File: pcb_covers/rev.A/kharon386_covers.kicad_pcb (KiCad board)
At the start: 2 copper layers, 134.6 x 63 mm, 2 parts

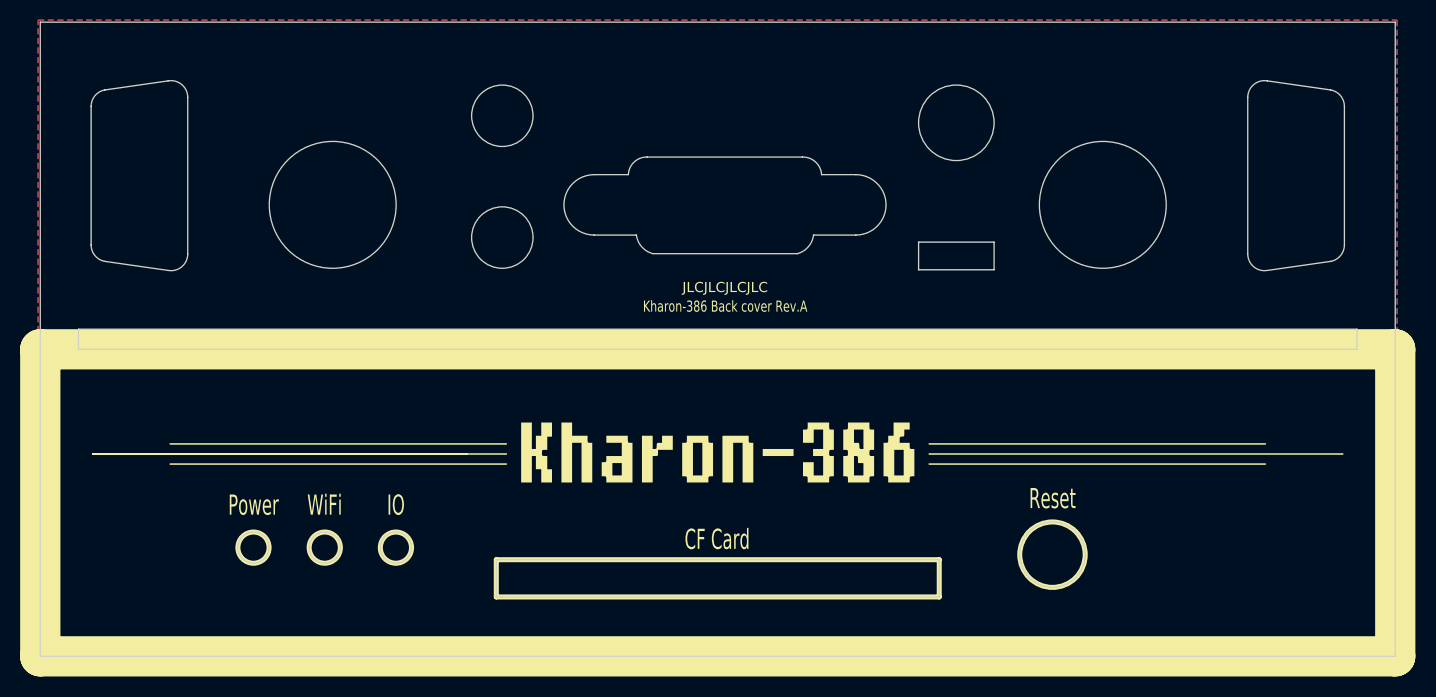
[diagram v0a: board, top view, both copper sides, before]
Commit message: pcb rev.A final version
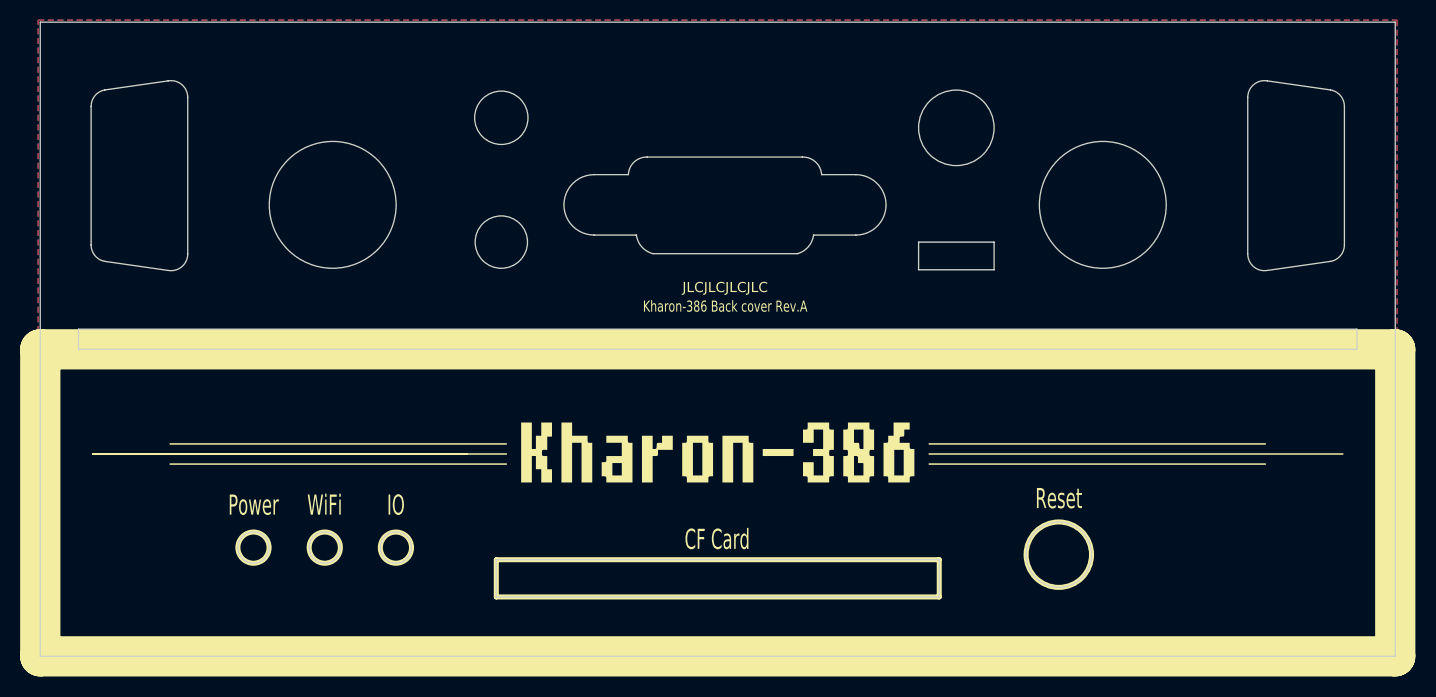
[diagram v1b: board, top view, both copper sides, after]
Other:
- outline, holes or cut-outs redrawn
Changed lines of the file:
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@@
   (gr_line (start 132.217828 76.65) (end 135.617828 76.65) (layer "B.SilkS") (width 0.5))
   (gr_arc (start 158.217828 76.65) (mid 161.21783 79.65) (end 158.217828 82.65) (layer "B.SilkS") (width 0.5))
-  (gr_circle (center 123.1 70.8) (end 126.15 70.8) (layer "B.SilkS") (width 0.5) (fill none))
+  (gr_circle (center 123 71) (end 125.65 71) (layer "B.SilkS") (width 0.5) (fill none))
   (gr_line (start 197.14969 84.529483) (end 197.14969 68.970509) (layer "B.SilkS") (width 0.5))
   (gr_arc (start 197.14969 68.970509) (mid 197.742659 67.698865) (end 199.097944 67.33573) (layer "B.SilkS") (width 0.5))
   (gr_arc (start 82.25 69.869781) (mid 82.638365 68.802753) (end 83.621743 68.235001) (layer "B.SilkS") (width 0.5))
-  (gr_circle (center 168.2 71.5) (end 171.95 71.5) (layer "B.SilkS") (width 0.5) (fill none))
+  (gr_circle (center 168.2 72) (end 171.95 72) (layer "B.SilkS") (width 0.5) (fill none))
   (gr_line (start 83.621744 85.265) (end 89.901744 86.164268) (layer "B.SilkS") (width 0.5))
-  (gr_circle (center 123.1 82.9) (end 126.15 82.9) (layer "B.SilkS") (width 0.5) (fill none))
+  (gr_circle (center 123 83.35) (end 125.6 83.35) (layer "B.SilkS") (width 0.5) (fill none))
   (gr_line (start 137.492828 74.9) (end 152.907172 74.9) (layer "B.SilkS") (width 0.5))
   (gr_line (start 138.053367 84.5) (end 152.417831 84.499999) (layer "B.SilkS") (width 0.5))
@@
   (gr_arc (start 205.377947 68.234995) (mid 206.361339 68.802744) (end 206.74969 69.869777) (layer "B.SilkS") (width 0.5))
   (gr_line (start 165.5 103.4) (end 198.9 103.4) (layer "F.SilkS") (width 0.15))
-  (gr_circle (center 177.75 114.4) (end 181 114.4) (layer "F.SilkS") (width 0.5) (fill none))
+  (gr_circle (center 178.38 114.4) (end 181.63 114.4) (layer "F.SilkS") (width 0.5) (fill none))
   (gr_line (start 123.5 104.4) (end 82.4 104.4) (layer "F.SilkS") (width 0.15))
   (gr_rect (start 77.2 94) (end 211.8 124.5) (layer "F.SilkS") (width 4) (fill none))
@@
   (gr_line (start 94.5 75.4) (end 194.5 75.4) (layer "Eco1.User") (width 0.015))
   (gr_circle (center 201.95 89.235) (end 203.35 89.235) (layer "Eco1.User") (width 0.1) (fill none))
-  (gr_circle (center 123.1 70.8) (end 126.15 70.8) (layer "Edge.Cuts") (width 0.1) (fill none))
+  (gr_circle (center 123 71) (end 125.65 71) (layer "Edge.Cuts") (width 0.1) (fill none))
   (gr_arc (start 197.14969 68.970509) (mid 197.742659 67.698865) (end 199.097944 67.33573) (layer "Edge.Cuts") (width 0.1))
   (gr_arc (start 83.621743 85.265001) (mid 82.638365 84.697247) (end 82.25 83.630219) (layer "Edge.Cuts") (width 0.1))
@@
   (gr_line (start 83.621744 68.235) (end 89.901744 67.335732) (layer "Edge.Cuts") (width 0.1))
   (gr_line (start 211.8 124.5) (end 77.2 124.5) (layer "Edge.Cuts") (width 0.1))
-  (gr_circle (center 168.2 71.5) (end 171.95 71.5) (layer "Edge.Cuts") (width 0.1) (fill none))
+  (gr_circle (center 168.2 72) (end 171.95 72) (layer "Edge.Cuts") (width 0.1) (fill none))
   (gr_line (start 154.817828 76.65) (end 158.217828 76.65) (layer "Edge.Cuts") (width 0.1))
   (gr_arc (start 91.85 84.529487) (mid 91.257029 85.801122) (end 89.901746 86.164266) (layer "Edge.Cuts") (width 0.1))
@@
   (gr_line (start 205.377946 68.234996) (end 199.097946 67.335728) (layer "Edge.Cuts") (width 0.1))
   (gr_line (start 197.14969 84.529483) (end 197.14969 68.970509) (layer "Edge.Cuts") (width 0.1))
-  (gr_circle (center 123.1 82.9) (end 126.15 82.9) (layer "Edge.Cuts") (width 0.1) (fill none))
+  (gr_circle (center 123 83.35) (end 125.6 83.35) (layer "Edge.Cuts") (width 0.1) (fill none))
   (gr_circle (center 182.75 79.65) (end 189.05 79.65) (layer "Edge.Cuts") (width 0.1) (fill none))
   (gr_arc (start 154.017828 82.65) (mid 153.496296 83.81584) (end 152.417831 84.499999) (layer "Edge.Cuts") (width 0.1))
@@
   (gr_arc (start 138.053367 84.5) (mid 136.953378 83.82451) (end 136.417828 82.65) (layer "Edge.Cuts") (width 0.1))
   (gr_arc (start 152.907172 74.9) (mid 154.216892 75.388074) (end 154.817828 76.65) (layer "Edge.Cuts") (width 0.1))
-  (gr_circle (center 177.75 114.4) (end 181 114.4) (layer "Edge.Cuts") (width 0.1) (fill none))
+  (gr_circle (center 178.38 114.4) (end 181.63 114.4) (layer "Edge.Cuts") (width 0.1) (fill none))
   (gr_circle (center 105.46 113.7) (end 107.01 113.7) (layer "Edge.Cuts") (width 0.1) (fill none))
   (gr_rect (start 164.45 83.35) (end 171.95 86.1) (layer "Edge.Cuts") (width 0.1) (fill none))
@@
   (gr_line (start 132.217828 82.65) (end 136.417828 82.65) (layer "Edge.Cuts") (width 0.1))
   (gr_line (start 132.217828 76.65) (end 135.617828 76.65) (layer "Edge.Cuts") (width 0.1))
-  (gr_text "5.1V 2.5A" (at 168.2 81.45) (layer "B.SilkS")
+  (gr_text "5.1V 2.5A" (at 168.2 81.25) (layer "B.SilkS")
     (effects (font (size 2 1.2) (thickness 0.2)) (justify mirror))
   )
@@
     (effects (font (size 1.1 0.8) (thickness 0.14)) (justify mirror))
   )
-  (gr_text "Power" (at 168.2 65.7) (layer "B.SilkS")
+  (gr_text "Power" (at 168.2 66.2) (layer "B.SilkS")
     (effects (font (size 2 1.2) (thickness 0.2)) (justify mirror))
   )
@@
     (effects (font (size 2 1.2) (thickness 0.2)) (justify mirror))
   )
-  (gr_text "Line In" (at 123.1 65.7) (layer "B.SilkS")
+  (gr_text "Line In" (at 123.1 66.2) (layer "B.SilkS")
     (effects (font (size 2 1.2) (thickness 0.2)) (justify mirror))
   )
-  (gr_text "Line Out" (at 123.1 77.85) (layer "B.SilkS")
+  (gr_text "Line Out" (at 123 78.8) (layer "B.SilkS")
     (effects (font (size 2 1.2) (thickness 0.2)) (justify mirror))
   )
@@
     (effects (font (size 2 1.2) (thickness 0.2)) (justify mirror))
   )
-  (gr_text "VGA" (at 145.407828 73.1) (layer "B.SilkS")
+  (gr_text "VGA" (at 145.407828 72.9) (layer "B.SilkS")
     (effects (font (size 2 1.2) (thickness 0.2)) (justify mirror))
   )
@@
     (effects (font (size 1.1 0.8) (thickness 0.14)))
   )
-  (gr_text "Reset" (at 177.75 108.85) (layer "F.SilkS")
+  (gr_text "Reset" (at 178.38 108.85) (layer "F.SilkS")
     (effects (font (size 2 1.2) (thickness 0.2)))
   )
